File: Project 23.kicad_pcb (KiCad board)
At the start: 2 copper layers, 62 x 42 mm, 47 parts, among them J11 SRX 1, J12 SRX 2, J13 SWD, J21 Batt, J61 USB_Micro, M1 Hole_M2, M2 Hole_M2, Q51 Si2315, SW11 UI_Btn, SW12 PWR_BTN, U1 STM32F103C8T7, U2 MCP73811, U3 NCP551, U4 NCP1402, U5 oled, Y11 8 MHz

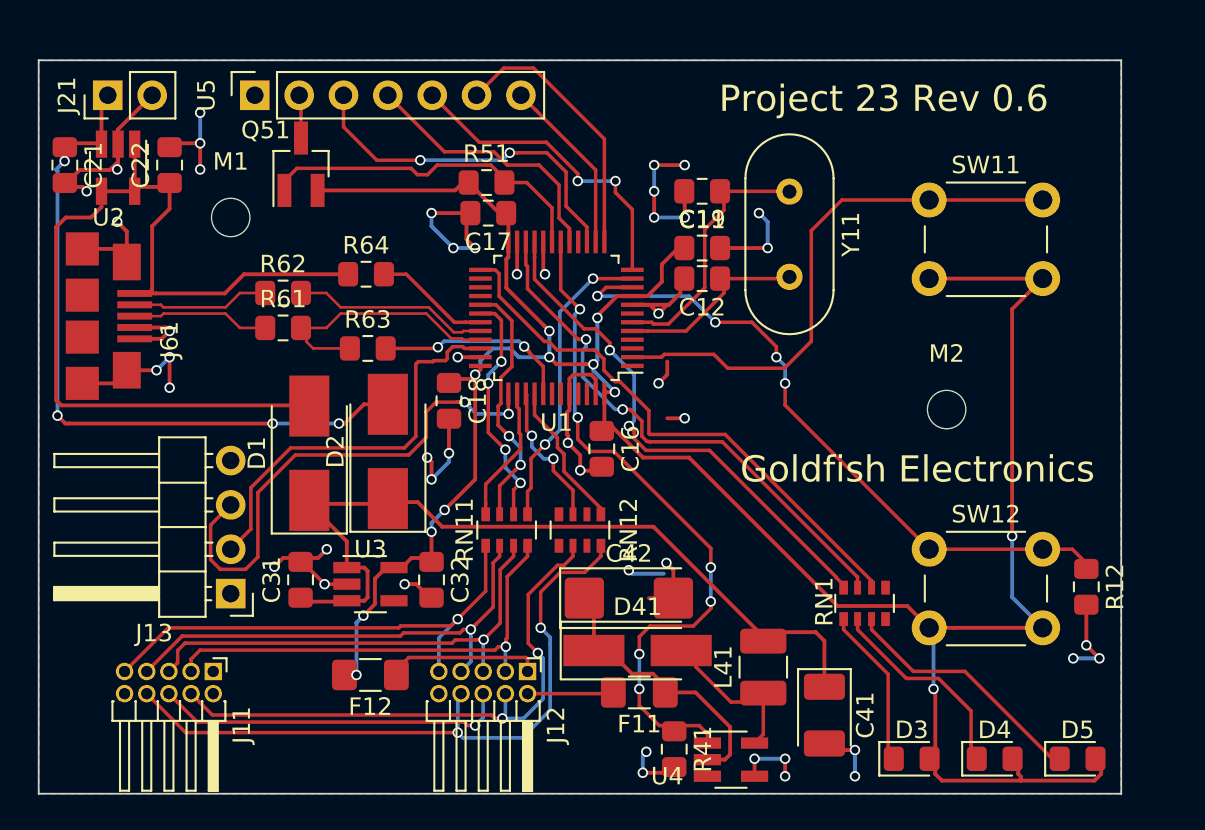
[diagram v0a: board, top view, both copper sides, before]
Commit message: Generated up to date gerber
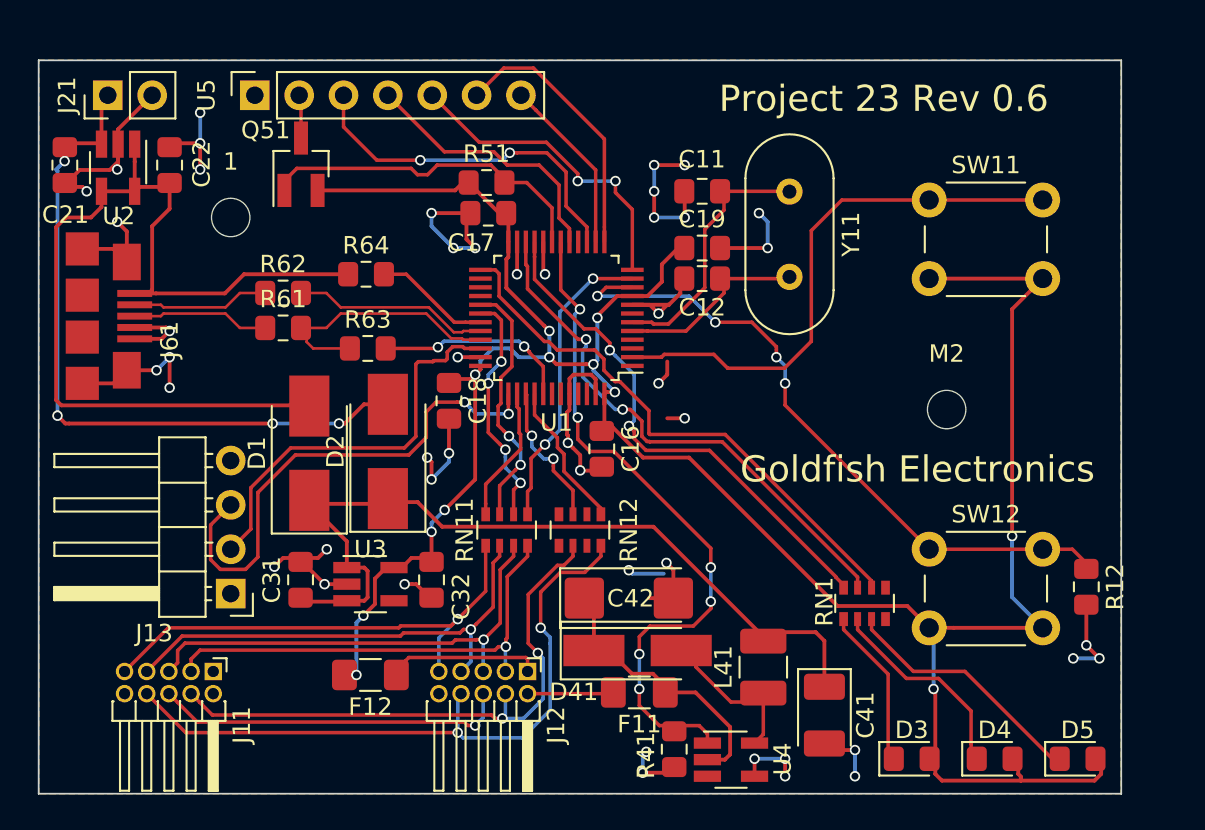
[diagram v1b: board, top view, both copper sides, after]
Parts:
- renumbered M1 to 1
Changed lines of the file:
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@@
     (38 B.Mask user)
     (39 F.Mask user)
-    (40 Dwgs.User user)
-    (41 Cmts.User user)
-    (42 Eco1.User user)
+    (40 Dwgs.User user hide)
+    (41 Cmts.User user hide)
+    (42 Eco1.User user hide)
     (43 Eco2.User user)
     (44 Edge.Cuts user)
     (45 Margin user)
-    (46 B.CrtYd user)
-    (47 F.CrtYd user)
-    (48 B.Fab user)
-    (49 F.Fab user)
+    (46 B.CrtYd user hide)
+    (47 F.CrtYd user hide)
+    (48 B.Fab user hide)
+    (49 F.Fab user hide)
   )
   (setup
@@
     (visible_elements 7FFFFFFF)
     (pcbplotparams
-      (layerselection 0x01020_7ffffffe)
+      (layerselection 0x010f0_ffffffff)
       (usegerberextensions true)
       (usegerberattributes false)
@@
       (padsonsilk false)
       (subtractmaskfromsilk false)
-      (outputformat 4)
+      (outputformat 1)
       (mirror false)
       (drillshape 0)
       (scaleselection 1)
-      (outputdirectory ""))
+      (outputdirectory "Gerber/"))
   )
   (net 0 "")
@@
       (net 6 VBUS))
   )
-  (module MountingHole:MountingHole_2.2mm_M2 (layer F.Cu)
+  (module MountingHole:MountingHole_2.2mm_M2 locked (layer F.Cu)
     (at 61 49)
     (descr "Mounting Hole 2.2mm, no annular, M2")
     (tags "mounting hole 2.2mm no annular m2")
     (attr virtual)
-    (fp_text reference M1 (at 0 -3.2) (layer F.SilkS)
+    (fp_text reference 1 (at 0 -3.2) (layer F.SilkS)
       (effects (font (size 1 1) (thickness 0.15)))
     )
@@
     (pad 1 np_thru_hole circle (at 0 0) (size 2.2 2.2) (drill 2.2) (layers *.Cu *.Mask))
   )
-  (module MountingHole:MountingHole_2.2mm_M2 (layer F.Cu)
+  (module MountingHole:MountingHole_2.2mm_M2 locked (layer F.Cu)
     (at 102 60)
     (descr "Mounting Hole 2.2mm, no annular, M2")
@@
     (tags "capacitor tantalum")
     (attr smd)
-    (fp_text reference C42 (at 0 -2.55) (layer F.SilkS)
+    (fp_text reference C42 (at 0.0962 0.0152) (layer F.SilkS)
       (effects (font (size 1 1) (thickness 0.15)))
     )
@@
     (tags "capacitor handsolder")
     (attr smd)
-    (fp_text reference C11 (at 0 -1.65 180) (layer F.SilkS)
+    (fp_text reference C11 (at 0.0144 1.8308 180) (layer F.SilkS)
       (effects (font (size 1 1) (thickness 0.15)))
     )
@@
     (tags "capacitor handsolder")
     (attr smd)
-    (fp_text reference C17 (at 0 -1.65 180) (layer F.SilkS)
+    (fp_text reference C17 (at 0.9724 -1.6944 180) (layer F.SilkS)
       (effects (font (size 1 1) (thickness 0.15)))
     )
@@
     (tags "capacitor handsolder")
     (attr smd)
-    (fp_text reference C21 (at 0 -1.65 270) (layer F.SilkS)
+    (fp_text reference C21 (at 2.8442 -0.0366) (layer F.SilkS)
       (effects (font (size 1 1) (thickness 0.15)))
     )
@@
     (tags "capacitor handsolder")
     (attr smd)
-    (fp_text reference C22 (at 0 -1.65 90) (layer F.SilkS)
+    (fp_text reference C22 (at 0.0514 1.8344 90) (layer F.SilkS)
       (effects (font (size 1 1) (thickness 0.15)))
     )
@@
     (tags "capacitor handsolder")
     (attr smd)
-    (fp_text reference C32 (at 0 -1.65 270) (layer F.SilkS)
+    (fp_text reference C32 (at 0.9636 -1.6934 270) (layer F.SilkS)
       (effects (font (size 1 1) (thickness 0.15)))
     )
@@
     (tags "Diode SMA (DO-214AC) Handsoldering")
     (attr smd)
-    (fp_text reference D41 (at 0 -2.5) (layer F.SilkS)
+    (fp_text reference D41 (at -3.655 2.3746) (layer F.SilkS)
       (effects (font (size 1 1) (thickness 0.15)))
     )
@@
     (tags "resistor handsolder")
     (attr smd)
-    (fp_text reference R41 (at 0 -1.65 270) (layer F.SilkS)
+    (fp_text reference R41 (at 0.3568 1.6148 270) (layer F.SilkS)
       (effects (font (size 1 1) (thickness 0.15)))
     )
@@
     (tags "SOT-23-5 hand-soldering")
     (attr smd)
-    (fp_text reference U2 (at 2.85 0.55) (layer F.SilkS)
+    (fp_text reference U2 (at 2.7704 -0.0346) (layer F.SilkS)
       (effects (font (size 1 1) (thickness 0.15)))
     )
@@
     (tags "SOT-23-5 hand-soldering")
     (attr smd)
-    (fp_text reference U4 (at -3.65 0.95) (layer F.SilkS)
-      (effects (font (size 1 1) (thickness 0.15)))
-    )
+    (fp_text reference U4 (at 2.9584 -0.04 90) (layer F.SilkS)
+      (effects (font (size 1 1) (thickness 0.15)))
+    )

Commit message: Completed V0.7 PCB Design
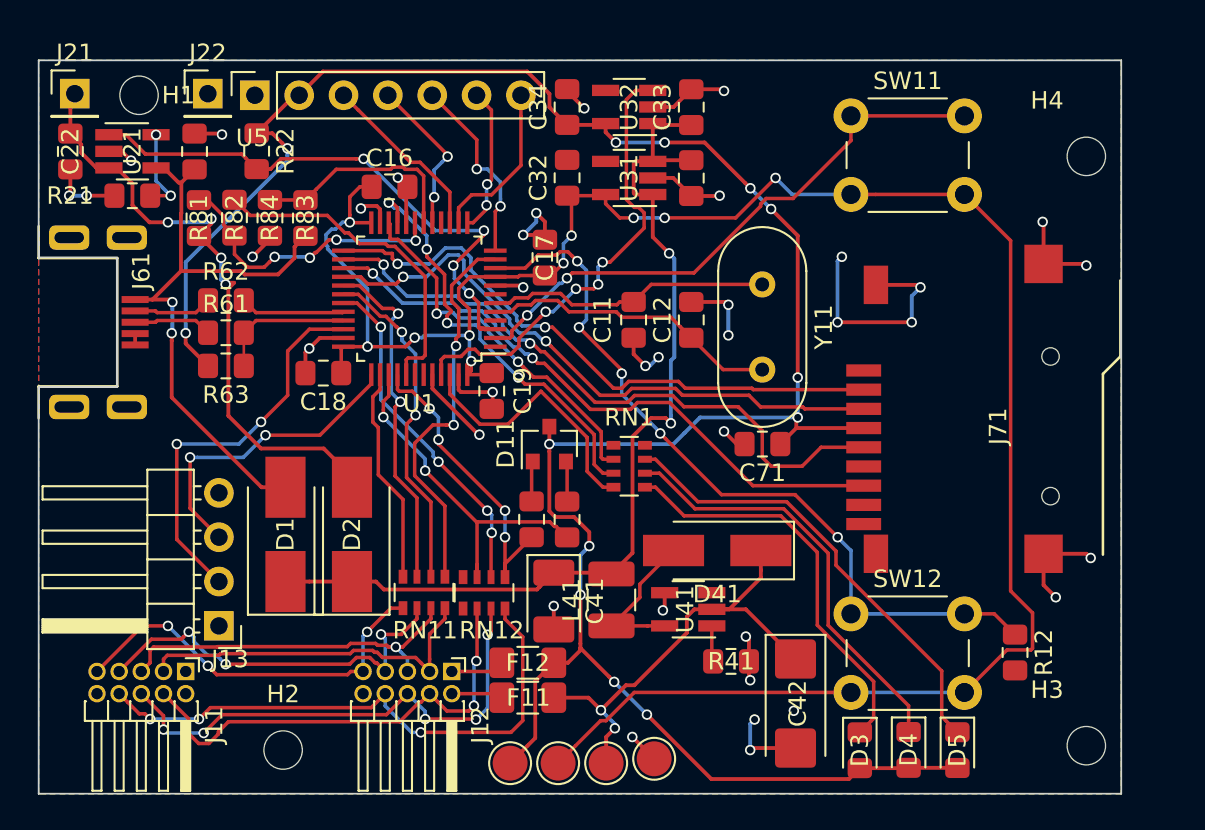
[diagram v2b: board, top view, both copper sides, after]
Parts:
- removed 1, M2: Hole_M2, MountingHole:MountingHole_2.2mm_M2
- removed Q51: Si2315, Package_TO_SOT_SMD:SOT-23_Handsoldering
- removed R51, R64: 10k, Resistor_SMD:R_0805_2012Metric_Pad1.15x1.40mm_HandSolder
- removed U2: MCP73811, Package_TO_SOT_SMD:SOT-23-5_HandSoldering
- removed U3: NCP551, Package_TO_SOT_SMD:SOT-23-5_HandSoldering
- removed U4: NCP1402, Package_TO_SOT_SMD:SOT-23-5_HandSoldering
- added C33: 1uF, Capacitor_SMD:C_0805_2012Metric_Pad1.15x1.40mm_HandSolder, F.Cu at (87.4, 42.7)
- added C34: 1uF, Capacitor_SMD:C_0805_2012Metric_Pad1.15x1.40mm_HandSolder, F.Cu at (80.3, 42.7)
- added C71: 1uF, Capacitor_SMD:C_0805_2012Metric_Pad1.15x1.40mm_HandSolder, F.Cu at (91.4, 62.0)
- added D11: MMBD1205, Package_TO_SOT_SMD:SOT-23, F.Cu at (79.2, 62.0)
- added H1: M2, MountingHole:MountingHole_2.2mm_M2, F.Cu at (55.8, 42.0)
- added H2: M2, MountingHole:MountingHole_2.2mm_M2, F.Cu at (64.0, 79.5)
- added H3: M2, MountingHole:MountingHole_2.2mm_M2, F.Cu at (107.8, 79.2)
- added H4: M2, MountingHole:MountingHole_2.2mm_M2, F.Cu at (107.8, 45.5)
- added J22: BATT-, Connector_PinHeader_2.54mm:PinHeader_1x01_P2.54mm_Vertical, F.Cu at (59.7, 41.9)
- added J71: Micro_SD_Card_Det, Project 23:micro sd holder, F.Cu at (108.0, 61.0)
- added R15: 10k, Resistor_SMD:R_0805_2012Metric_Pad1.15x1.40mm_HandSolder, F.Cu at (80.3, 66.3)
- added R16: 10k, Resistor_SMD:R_0805_2012Metric_Pad1.15x1.40mm_HandSolder, F.Cu at (78.2, 66.3)
- added R21: 10k, Resistor_SMD:R_0805_2012Metric_Pad1.15x1.40mm_HandSolder, F.Cu at (55.4, 47.8)
- added R22: 10k, Resistor_SMD:R_0805_2012Metric_Pad1.15x1.40mm_HandSolder, F.Cu at (62.5, 45.2)
- added R81: 10k, Resistor_SMD:R_0805_2012Metric_Pad1.15x1.40mm_HandSolder, F.Cu at (59.2, 49.0)
- added R82: 10k, Resistor_SMD:R_0805_2012Metric_Pad1.15x1.40mm_HandSolder, F.Cu at (61.2, 49.0)
- added R83: 10k, Resistor_SMD:R_0805_2012Metric_Pad1.15x1.40mm_HandSolder, F.Cu at (65.3, 49.0)
- added R84: 10k, Resistor_SMD:R_0805_2012Metric_Pad1.15x1.40mm_HandSolder, F.Cu at (63.2, 49.0)
- added TP31: 3V3SB, TestPoint:TestPoint_Pad_D2.0mm, F.Cu at (79.8, 80.2)
- added TP32: 3V3, TestPoint:TestPoint_Pad_D2.0mm, F.Cu at (77.0, 80.2)
- added TP41: 5V, TestPoint:TestPoint_Pad_D2.0mm, F.Cu at (82.5, 80.2)
- added TP75: GND, TestPoint:TestPoint_Pad_D2.0mm, F.Cu at (85.2, 80.0)
- added U21: MCP73832, Package_TO_SOT_SMD:SOT-23-5_HandSoldering, F.Cu at (55.4, 45.2)
- added U31: NCP551, Package_TO_SOT_SMD:SOT-23-5_HandSoldering, F.Cu at (83.8, 46.7)
- added U32: MIC5504, Package_TO_SOT_SMD:SOT-23-5_HandSoldering, F.Cu at (83.8, 42.7)
- added U41: NCP1402, Package_TO_SOT_SMD:SOT-23-5_HandSoldering, F.Cu at (87.2, 71.4)
- J21: value Batt -> BATT +; footprint Connector_PinHeader_2.54mm:PinHeader_1x02_P2.54mm_Vertical -> Connector_PinHeader_2.54mm:PinHeader_1x01_P2.54mm_Vertical
- J61: footprint Project 23:usbMicro -> Project 23:microUsbSunken
- moved C31 32.1 mm to (87.4, 46.7), turned to 270 degrees
- moved C32 24.3 mm to (80.3, 46.7), turned to 90 degrees
- moved C16 19.3 mm to (70.1, 47.2), turned to 0 degrees
- moved C41 16.8 mm to (79.5, 71.0)
- moved RN1 15.6 mm to (83.8, 63.2), turned to 0 degrees
- moved C19 14.6 mm to (75.9, 58.9), turned to 270 degrees
- moved C42 11.3 mm to (93.3, 76.8), turned to 270 degrees
- moved L41 9.51 mm to (82.8, 70.9)
- moved F12 9.04 mm to (78.0, 74.5), turned to 0 degrees
- moved C11 8.35 mm to (84.1, 54.9), turned to 270 degrees
- moved R63 8.19 mm to (60.7, 57.5), turned to 180 degrees
- moved U1 7.93 mm to (71.8, 53.6)
- moved C21 7.47 mm to (58.9, 45.2), turned to 90 degrees
- moved C18 7.37 mm to (66.3, 57.9), turned to 180 degrees
- moved D41 7.32 mm to (88.9, 68.1), turned to 180 degrees
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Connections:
- C16 pad 1: +3V3 -> /3V3SB
- C17 pad 1: +3V3 -> /3V3SB
- C18 pad 1: +3V3 -> /3V3SB
- C19 pad 1: +3V3 -> /3V3SB
- C21 pad 1: +BATT -> VBUS
- C22 pad 1: VBUS -> +BATT
- C32 pad 1: +3V3 -> /3V3SB
- R41 pad 1: /Boost_En -> /PWR_EN
- R63 pad 2: /USB_PU -> +3V3
- RN12 pad 3: (no net) -> Net-(J11-Pad6)
- RN12 pad 6: (no net) -> /Trigger
- SW11 pad 2: +3V3 -> /3V3SB
- SW12 pad 2: +3V3 -> /3V3SB
- U1 pad 18: /Boost_En -> /VBus_Mon
- U1 pad 19: /OLED_En -> /Batt_Mon
- U1 pad 21: /Fwd_LED -> /Rev_LED
- U1 pad 22: /Rev_LED -> /Pwr_LED
- U1 pad 24: +3V3 -> /3V3SB
- U1 pad 25: /Pwr_LED -> /SS2
- U1 pad 26: (no net) -> /SCK2
- U1 pad 27: (no net) -> /MISO2
- U1 pad 28: (no net) -> /MOSI2
- U1 pad 3: (no net) -> /Stat
- U1 pad 31: /VBus_Sense -> /Trigger
- U1 pad 36: +3V3 -> /3V3SB
- U1 pad 41: /USB_PU -> /R_DIV_En
- U1 pad 45: (no net) -> /PWR_En
- U1 pad 46: (no net) -> /Fwd_LED
- U1 pad 48: +3V3 -> /3V3SB
- U1 pad 9: +3V3 -> /3V3SB
- U5 pad 2: Net-(Q51-Pad3) -> +3V3
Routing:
- net /3V3SB: track 0.00 -> 122.3 mm, vias 0 -> 10
- net /Boost_En: track 39.5 -> 0.00 mm, vias 6 -> 0
- net /SCK2: track 0.00 -> 36.8 mm, vias 0 -> 2
- net /MISO2: track 0.00 -> 35.4 mm, vias 0 -> 2
- net /MOSI2: track 0.00 -> 35.2 mm, vias 0 -> 2
- net /SS2: track 0.00 -> 34.9 mm, vias 0 -> 2
- net /Stat: track 0.00 -> 33.1 mm, vias 0 -> 4
- net /PWR_En: track 0.00 -> 26.3 mm, vias 0 -> 4
- net GND: track 110.7 -> 86.0 mm, vias 47 -> 37
- net VBUS: track 55.0 -> 35.1 mm, vias 0 -> 2
- net /Trigger: track 0.00 -> 19.7 mm, vias 0 -> 4
- net /OLED_En: track 19.5 -> 0.00 mm
- net /R_DIV_En: track 0.00 -> 19.3 mm
- net /Batt_Mon: track 0.00 -> 16.7 mm, vias 0 -> 4
- net /Fwd_LED: track 30.2 -> 15.4 mm, vias 2 -> 0
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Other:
- outline, holes or cut-outs redrawn
- board text removed: "Goldfish Electronics"
- board text removed: "Project 23 Rev 0.6"
